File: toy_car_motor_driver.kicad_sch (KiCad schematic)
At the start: 15 parts, among them J1 Conn_01x06_Pin, J3 Conn_01x02_Pin, J4 Screw_Terminal_01x02, J5 Screw_Terminal_01x02, J6 Screw_Terminal_01x02, SW1 SW_DIP_x04, U1 L293D

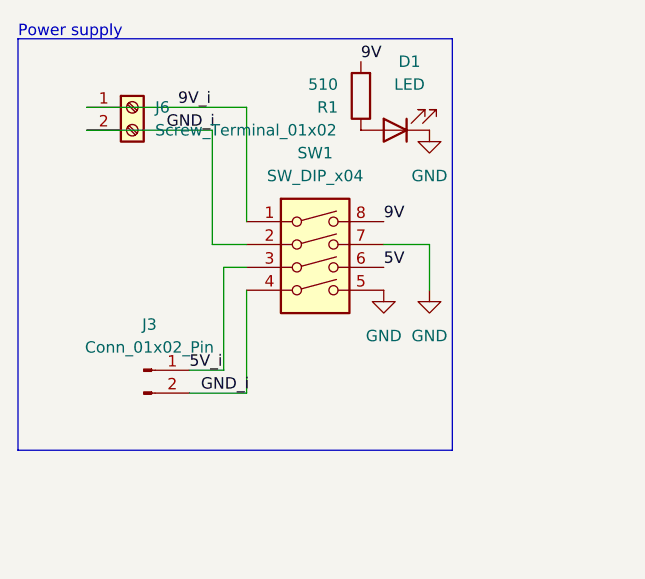
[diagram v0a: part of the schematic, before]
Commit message: Updated pcb
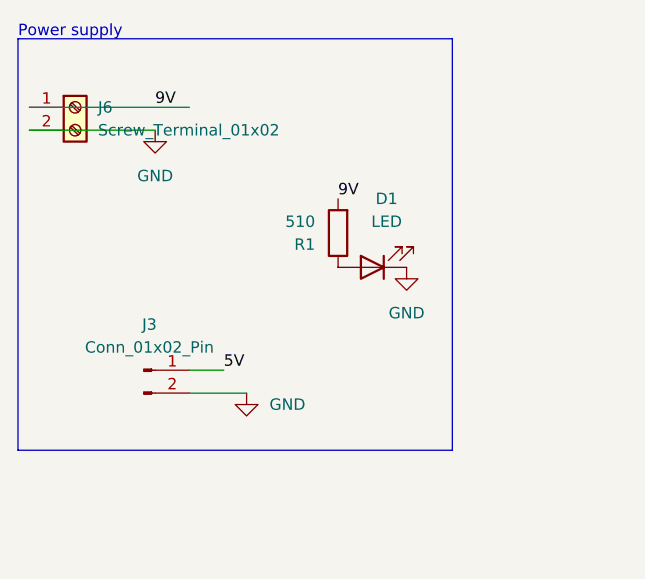
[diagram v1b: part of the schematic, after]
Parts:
- removed SW1: SW_DIP_x04, Package_DIP:DIP-8_W7.62mm, symbol Switch:SW_DIP_x04
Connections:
- net 5V_i is gone; now on net 5V: J3.1 (Pin_1)
- net 9V_i is gone; now on net 9V: J6.1 (Pin_1)
- net GND_i is gone; now on net GND: J3.2 (Pin_2), J6.2 (Pin_2)
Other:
- moved on the sheet: D1, J6, R1
